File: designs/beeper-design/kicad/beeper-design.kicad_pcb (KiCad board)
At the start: 4 copper layers, 27.5 x 19 mm, 100 parts

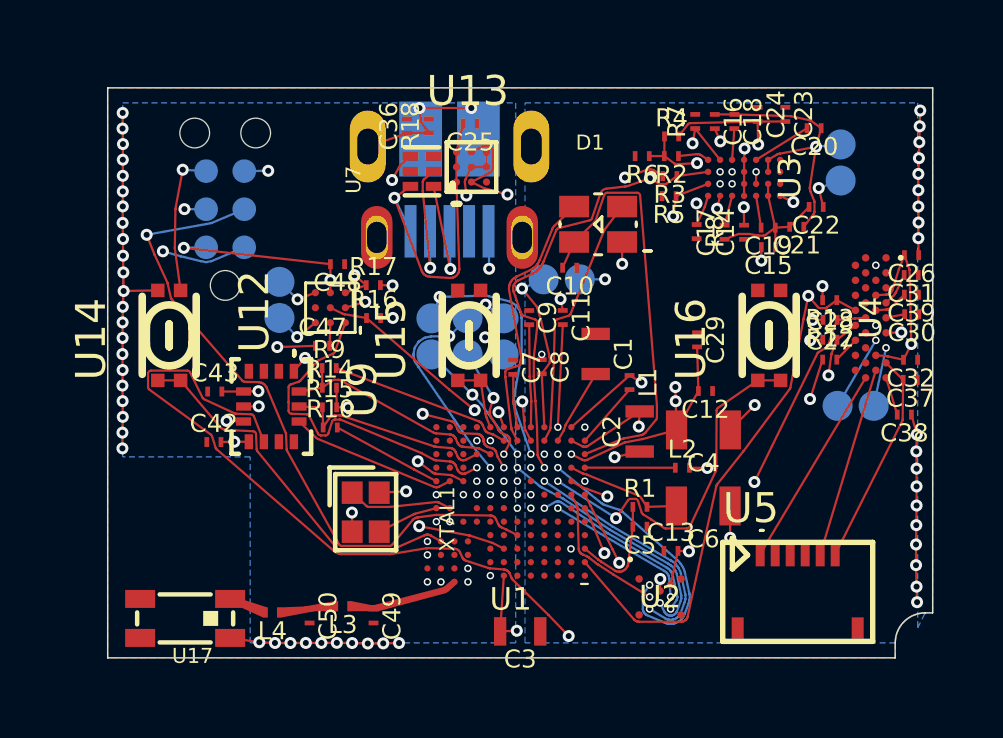
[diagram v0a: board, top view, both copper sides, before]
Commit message: another export
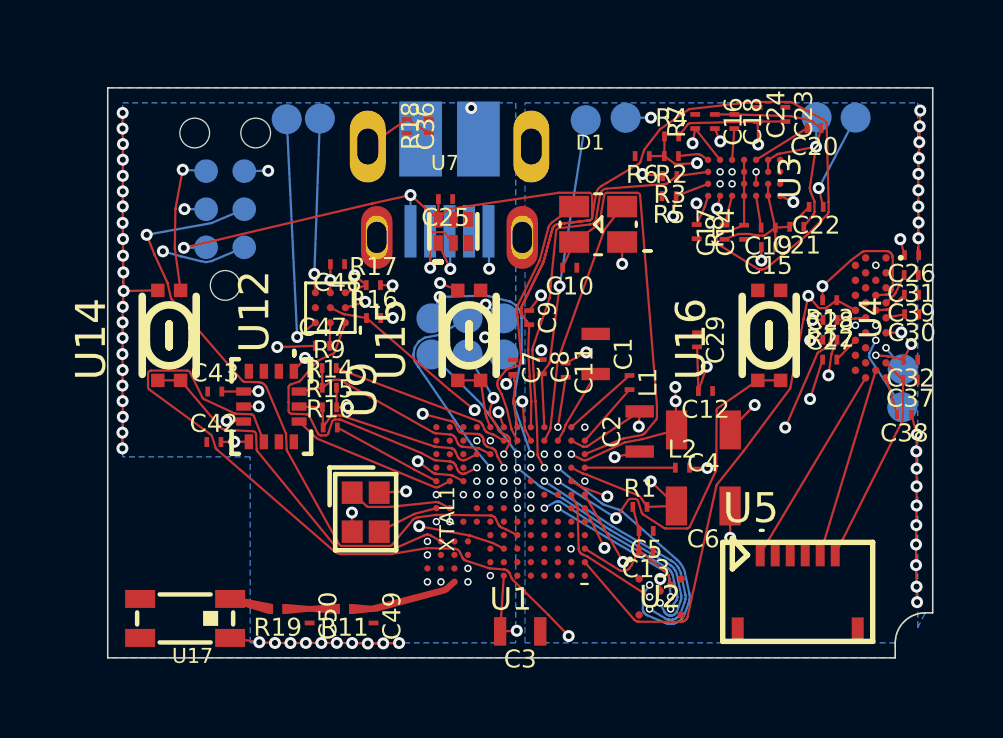
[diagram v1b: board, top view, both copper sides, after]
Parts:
- removed L3: 470n, beeper-design:Pkg0201_13
- removed L4: 470n, beeper-design:Pkg0201_36
- removed U13: ~, beeper-design:LP_6
- added R11: 0R, beeper-design:Pkg0201_53, F.Cu at (133.6, 115.9)
- added R19: 0R, beeper-design:Pkg0201_19, F.Cu at (131.4, 115.9)
- C10: footprint beeper-design:Pkg0201_37 -> beeper-design:Pkg0201_18
- C11: footprint beeper-design:Pkg0201_29 -> beeper-design:Pkg0201_13
- C12: footprint beeper-design:Pkg0201_48 -> beeper-design:Pkg0201_31
- C13: footprint beeper-design:Pkg0201_51 -> beeper-design:Pkg0201_34
- C14: footprint beeper-design:Pkg0201_18 -> beeper-design:Pkg0201_2
- C15: footprint beeper-design:Pkg0201_11 -> beeper-design:Pkg0201_51
- C16: footprint beeper-design:Pkg0201_27 -> beeper-design:Pkg0201_12
- C17: footprint beeper-design:Pkg0201_40 -> beeper-design:Pkg0201_25
- C18: footprint beeper-design:Pkg0201_53 -> beeper-design:Pkg0201_37
- C19: footprint beeper-design:Pkg0201_10 -> beeper-design:Pkg0201_49
- C20: footprint beeper-design:Pkg0201_26 -> beeper-design:Pkg0201_10
- C21: footprint beeper-design:Pkg0201_39 -> beeper-design:Pkg0201_23
- C22: footprint beeper-design:Pkg0201_52 -> beeper-design:Pkg0201_35
- C23: footprint beeper-design:Pkg0201_9 -> beeper-design:Pkg0201_48
- C24: footprint beeper-design:Pkg0201_23 -> beeper-design:Pkg0201_7
- C25: footprint beeper-design:Pkg0201_16 -> beeper-design:Pkg0201_22
- C26: footprint beeper-design:Pkg0201_19 -> beeper-design:Pkg0201_42
- C27: footprint beeper-design:Pkg0201_33 -> beeper-design:Pkg0201_4
- C28: footprint beeper-design:Pkg0201_46 -> beeper-design:Pkg0201_47
- C29: footprint beeper-design:Pkg0201_3 -> beeper-design:Pkg0201_30
- C30: footprint beeper-design:Pkg0201_43 -> beeper-design:Pkg0201_16
- C31: footprint beeper-design:Pkg0201 -> beeper-design:Pkg0201_29
- C32: footprint beeper-design:Pkg0201_12 -> beeper-design:Pkg0201_17
- C36: footprint beeper-design:Pkg0201_49 -> beeper-design:Pkg0201_33
- C37: footprint beeper-design:Pkg0201_17 -> beeper-design:Pkg0201_45
- C38: footprint beeper-design:Pkg0201_31 -> beeper-design:Pkg0201_3
- C39: footprint beeper-design:Pkg0201_28 -> beeper-design:Pkg0201_1
- C4: footprint beeper-design:Pkg0805 -> beeper-design:Pkg0805_1
- C42: footprint beeper-design:Pkg0201_21 -> beeper-design:Pkg0201_50
- C43: footprint beeper-design:Pkg0201_34 -> beeper-design:Pkg0201_9
- C47: footprint beeper-design:Pkg0201_35 -> beeper-design:Pkg0201_11
- C48: footprint beeper-design:Pkg0201_47 -> beeper-design:Pkg0201_24
- C49: footprint beeper-design:Pkg0201_4 -> beeper-design:Pkg0201_44
- C5: footprint beeper-design:Pkg0201_24 -> beeper-design:Pkg0201_6
- C50: footprint beeper-design:Pkg0201_25 -> beeper-design:Pkg0201_8
- C6: footprint beeper-design:Pkg0805_1 -> beeper-design:Pkg0805
- C7: footprint beeper-design:Pkg0201_50 -> beeper-design:Pkg0201_32
- C8: footprint beeper-design:Pkg0201_6 -> beeper-design:Pkg0201_46
- C9: footprint beeper-design:Pkg0201_22 -> beeper-design:Pkg0201_5
- L1: footprint beeper-design:Pkg0201_1 -> beeper-design:Pkg0201_40
- L2: footprint beeper-design:Pkg0201_14 -> beeper-design:Pkg0201_54
- R1: footprint beeper-design:Pkg0201_44 -> beeper-design:Pkg0201_27
- R10: footprint beeper-design:Pkg0201_20 -> beeper-design:Pkg0201_52
- R12, R13: footprint beeper-design:Pkg0201_5 -> beeper-design:Pkg0201_36
- R14, R15: footprint beeper-design:Pkg0201_42 -> beeper-design:Pkg0201_20
- R16, R17: footprint beeper-design:Pkg0201_8 -> beeper-design:Pkg0201_39
- R18: footprint beeper-design:Pkg0201_38 -> beeper-design:Pkg0201_21
- R2: footprint beeper-design:Pkg0201_32 -> beeper-design:Pkg0201_15
- R3: footprint beeper-design:Pkg0201_30 -> beeper-design:Pkg0201_14
- R4: footprint beeper-design:Pkg0201_2 -> beeper-design:Pkg0201_41
- R5: footprint beeper-design:Pkg0201_15 -> beeper-design:Pkg0201
- R6: footprint beeper-design:Pkg0201_45 -> beeper-design:Pkg0201_28
- R7: footprint beeper-design:Pkg0201_41 -> beeper-design:Pkg0201_26
- R8: footprint beeper-design:Pkg0201_54 -> beeper-design:Pkg0201_38
- R9: footprint beeper-design:Pkg0201_7 -> beeper-design:Pkg0201_43
- U12: footprint beeper-design:LP_8 -> beeper-design:LP_7
- U3: footprint beeper-design:LP_7 -> beeper-design:LP_6
- moved TP1 6.63 mm to (131.7, 99.5)
- moved TP2 5.61 mm to (132.8, 99.5)
- moved TP12 5.60 mm to (143.0, 99.5)
- moved TP11 5.49 mm to (141.7, 99.6)
- moved ? 5.35 mm to (135.7, 115.5)
- moved ? 3.77 mm to (130.5, 115.7)
- moved ? 3.01 mm to (134.3, 115.9)
- moved C25 2.65 mm to (137.0, 102.2)
- moved U7 2.26 mm to (137.3, 103.3), turned to 0 degrees
- moved TP3 2.16 mm to (152.2, 109.1)
- moved TP13 2.15 mm to (150.7, 99.5)
- moved C11 1.76 mm to (141.0, 107.9)
- moved TP4 1.56 mm to (152.3, 107.9)
- moved ? 1.51 mm to (137.2, 115.1)
- moved TP14 1.21 mm to (149.4, 99.5)
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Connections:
- net mcu_dbg-m33_swdio renamed mcu_mcu-dbg-m33_swdio
- net mcu_mcu-uart_rx renamed mcu_conn-uart_rx
- net mcu_mcu-uart_tx renamed mcu_conn-uart_tx
- net mcu_q-i3c_sda renamed board-io_qsen-i3c_sda
- C11 pad 2: VDD1P8 -> VDDSYS
- C12 pad 2: VDD1P8 -> VDDSYS
- C13 pad 2: VDD1P8 -> V18F
- C14 pad 2: VDD1P8 -> VBUS
- C26 pad 2: VDD_IO -> VDD3P0
- C28 pad 2: VDD_IO -> VDD1P8P
- C29 pad 2: VDD1P8 -> VDDSYS
- C32 pad 2: VDD_IO -> VDD3P0
- C48 pad 2: VDD1P8 -> VDDSYS
- C6 pad 2: V18P -> VDD1P8P
- C9 pad 2: mcu_VBUS -> VBUS
- J1 pad 1: VDD1P8 -> VBUS
- L2 pad 2: VDD1P8 -> VDDSYS
- R1 pad 2: V18P -> VDD1P8P
- R12 pad 2: VDD1P8 -> VDD1P8P
- R13 pad 2: VDD1P8 -> VDD1P8P
- R16 pad 2: VDD1P8 -> VDDSYS
- R17 pad 2: VDD1P8 -> VDDSYS
- U1 pad J2: V18P -> VDD1P8P
- U1 pad M3: VDD1P8 -> VDDSYS
- U1 pad M5: mcu_VBUS -> VBUS
- U12 pad C2: VDD1P8 -> VDDSYS
- U2 pad B2: VDD1P8 -> V18F
- U3 pad D1: VDD1P8 -> VBUS
- U3 pad D2: VDD1P8 -> VBUS
- U3 pad D3: VDD1P8 -> VBUS
- U3 pad D4: VDD1P8 -> VBUS
- U3 pad F3: nAD-EN -> (no net)
- U4 pad A11: VDD1P8 -> VDDSYS
- U4 pad B14: VDD_IO -> VDD3P0
- U4 pad B6: VDD_IO -> VDD1P8P
- U4 pad D10: VDD_IO -> VDD3P0
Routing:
- net VBUS: track 10.9 -> 52.0 mm, vias 1 -> 2
- net VDD3P0: track 1.77 -> 28.2 mm, vias 0 -> 5
- net VDD1P8P: track 0.00 -> 22.8 mm, vias 0 -> 4
- net VDD_IO: track 11.3 -> 0.00 mm, vias 2 -> 0
- net nAD-EN: track 10.9 -> 0.00 mm, vias 3 -> 0
- net VDDSYS: track 0.00 -> 6.88 mm, vias 0 -> 7
- net VDD1P8: track 29.8 -> 23.1 mm, vias 19 -> 6
- net OUT+: track 1.64 -> 8.04 mm
- net VBAT: track 5.72 -> 10.4 mm
- net OUT-: track 1.47 -> 5.81 mm
- net V18P: track 3.88 -> 0.00 mm
- net mcu_VBUS: track 3.42 -> 0.00 mm
- net SHIELD: track 10.2 -> 7.91 mm, vias 2 -> 1
- net D-: track 20.3 -> 18.3 mm
- net cap_p1: track 1.42 -> 3.30 mm
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- added copper zone on In2.Cu, net VDDSYS
- removed copper zone on In2.Cu, net VDD1P8
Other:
- rule pad_to_mask_clearance: 0 -> 0.051
